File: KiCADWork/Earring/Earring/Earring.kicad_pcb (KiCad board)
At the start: 2 copper layers, 9.2 x 9.2 mm, 3 parts, among them J1 Screw_Terminal_01x02, J2 Screw_Terminal_01x01

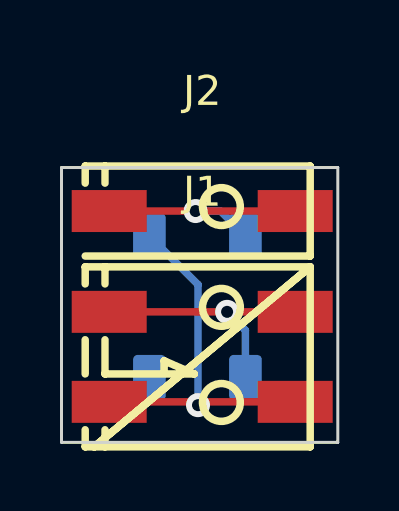
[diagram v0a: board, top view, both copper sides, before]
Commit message: Large Update
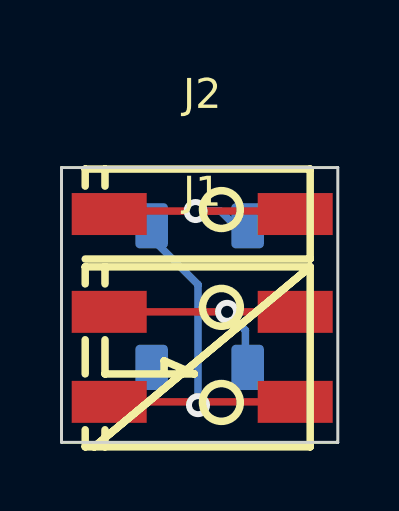
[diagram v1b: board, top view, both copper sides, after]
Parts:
- moved D1 0.35 mm to (170.7, 90.7)
- moved J2 0.10 mm to (170.8, 89.4)
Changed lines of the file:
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@@
   )
   (footprint "easyeda2kicad:CONN-SMD_custom1" (layer "F.Cu")
-    (at 170.77 89.3)
+    (at 170.77 89.4)
     (property "Sheetfile" "Earring.kicad_sch")
     (property "Sheetname" "")
@@
   )
   (footprint "easyeda2kicad:SOL320P540X170-4N" (layer "B.Cu")
-    (at 170.61 90.99 90)
+    (at 170.685 90.65 90)
     (property "Availability" "In Stock")
     (property "Check_prices" "https://www.snapeda.com/parts/2758/Adafruit+Industries+LLC/view-part/?ref=eda")

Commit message: Started mirror earrings and case
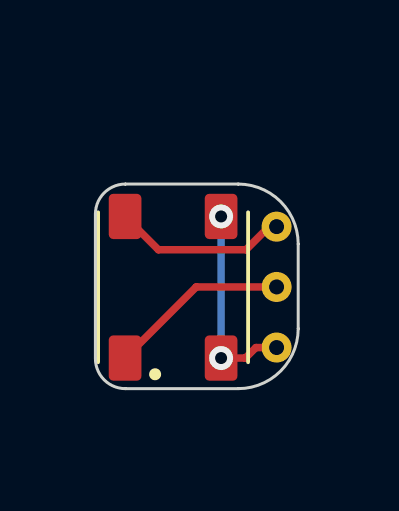
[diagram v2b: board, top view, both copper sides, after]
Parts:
- removed J1: Screw_Terminal_01x02, easyeda2kicad:CONN-SMD_2059-302
- removed J2: Screw_Terminal_01x01, easyeda2kicad:CONN-SMD_custom1
- added TP1: TestPoint, TestPoint:TestPoint_THTPad_D1.0mm_Drill0.5mm, B.Cu at (173.2, 88.3)
- added TP2: TestPoint, TestPoint:TestPoint_THTPad_D1.0mm_Drill0.5mm, B.Cu at (173.2, 90.3)
- added TP3: TestPoint, TestPoint:TestPoint_THTPad_D1.0mm_Drill0.5mm, B.Cu at (173.2, 92.3)
- D1: moved to F.Cu
- moved D1 0.94 mm to (169.8, 90.3)
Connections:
- D1 pad 2: unconnected-(D1-DOUT-Pad2) -> Net-(D1-DOUT)
- D1 pad 3: Net-(D1-VSS) -> Net-(D1-DOUT)
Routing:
- net Net-(D1-VSS): track 12.7 -> 0.00 mm, vias 1 -> 0
- net Net-(D1-DOUT): track 0.00 -> 6.97 mm, vias 0 -> 2
- net Net-(D1-VDD): track 8.66 -> 6.02 mm, vias 1 -> 0
- net Net-(D1-DIN): track 8.20 -> 5.92 mm, vias 1 -> 0
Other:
- board size 9.2 x 9.2 mm -> 6.8 x 6.8 mm
